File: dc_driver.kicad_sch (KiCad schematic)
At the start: 30 parts, among them J1 Conn_01x02, J10 Conn_01x02, J11 Conn_01x02, J12 Conn_01x02, J13 Conn_01x02, J14 Conn_01x02, J15 Conn_01x02, J2 Conn_01x02, J3 Conn_01x02, J4 Conn_01x02, J5 Conn_01x02, J6 Conn_01x02, J7 Conn_01x02, J8 Conn_01x02, J9 Conn_01x02, U4 MX1508, U5 MX1508, U6 MX1508

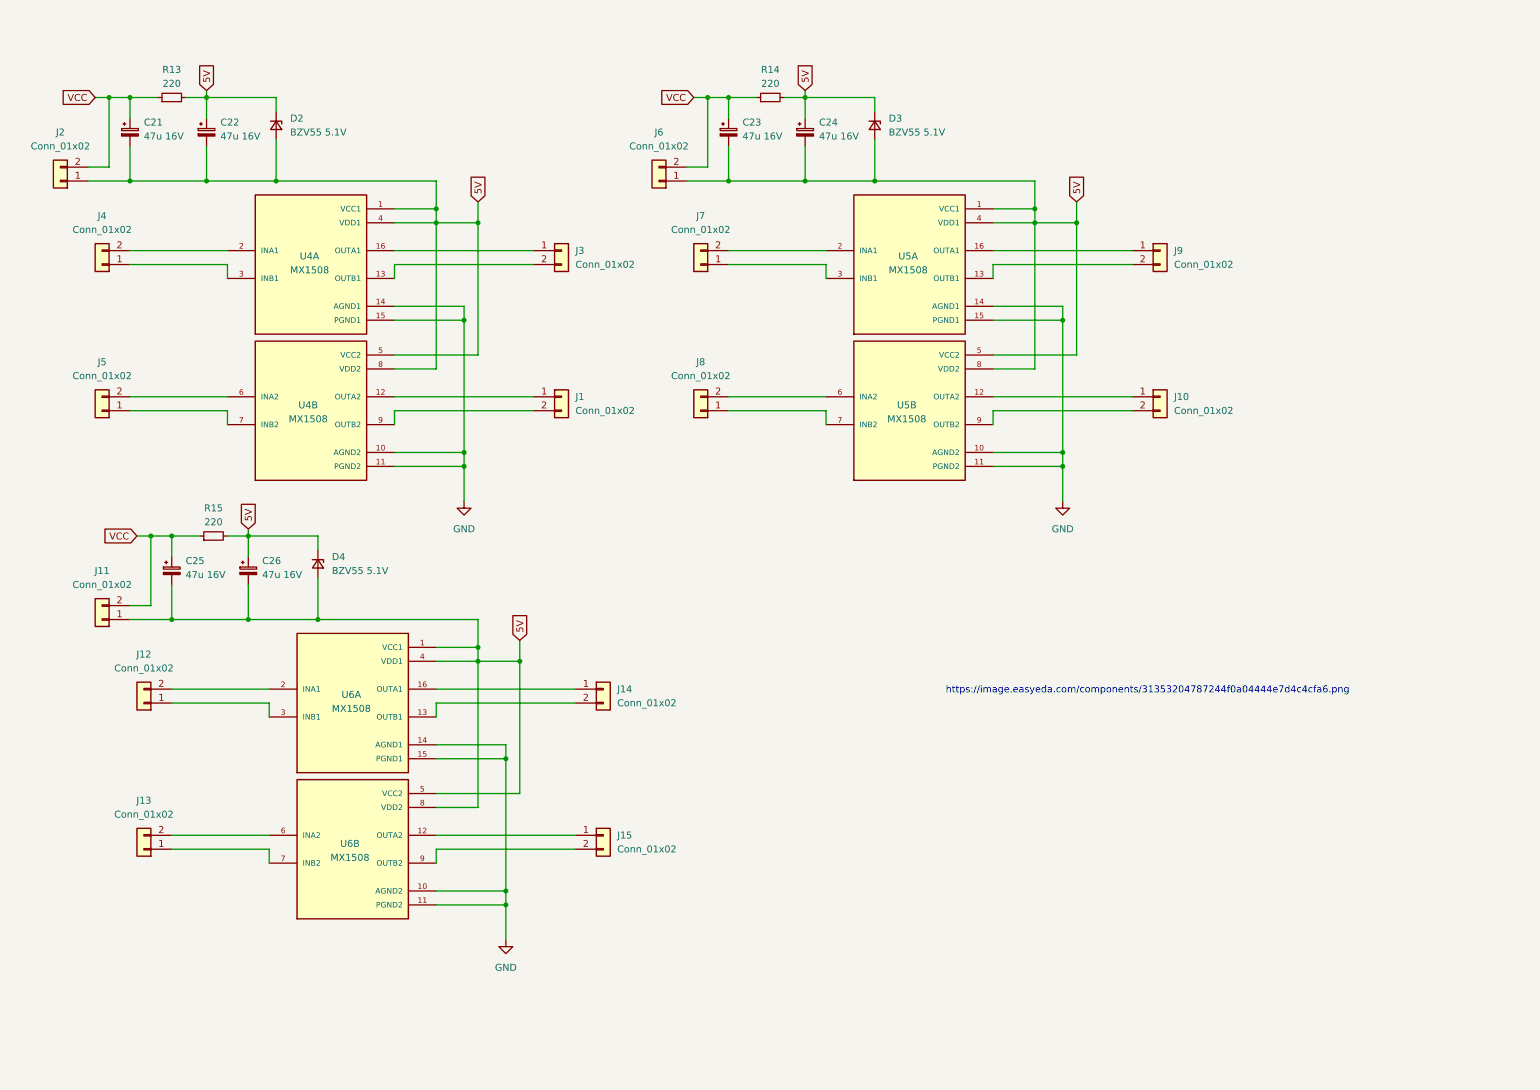
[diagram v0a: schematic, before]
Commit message: stm32 added
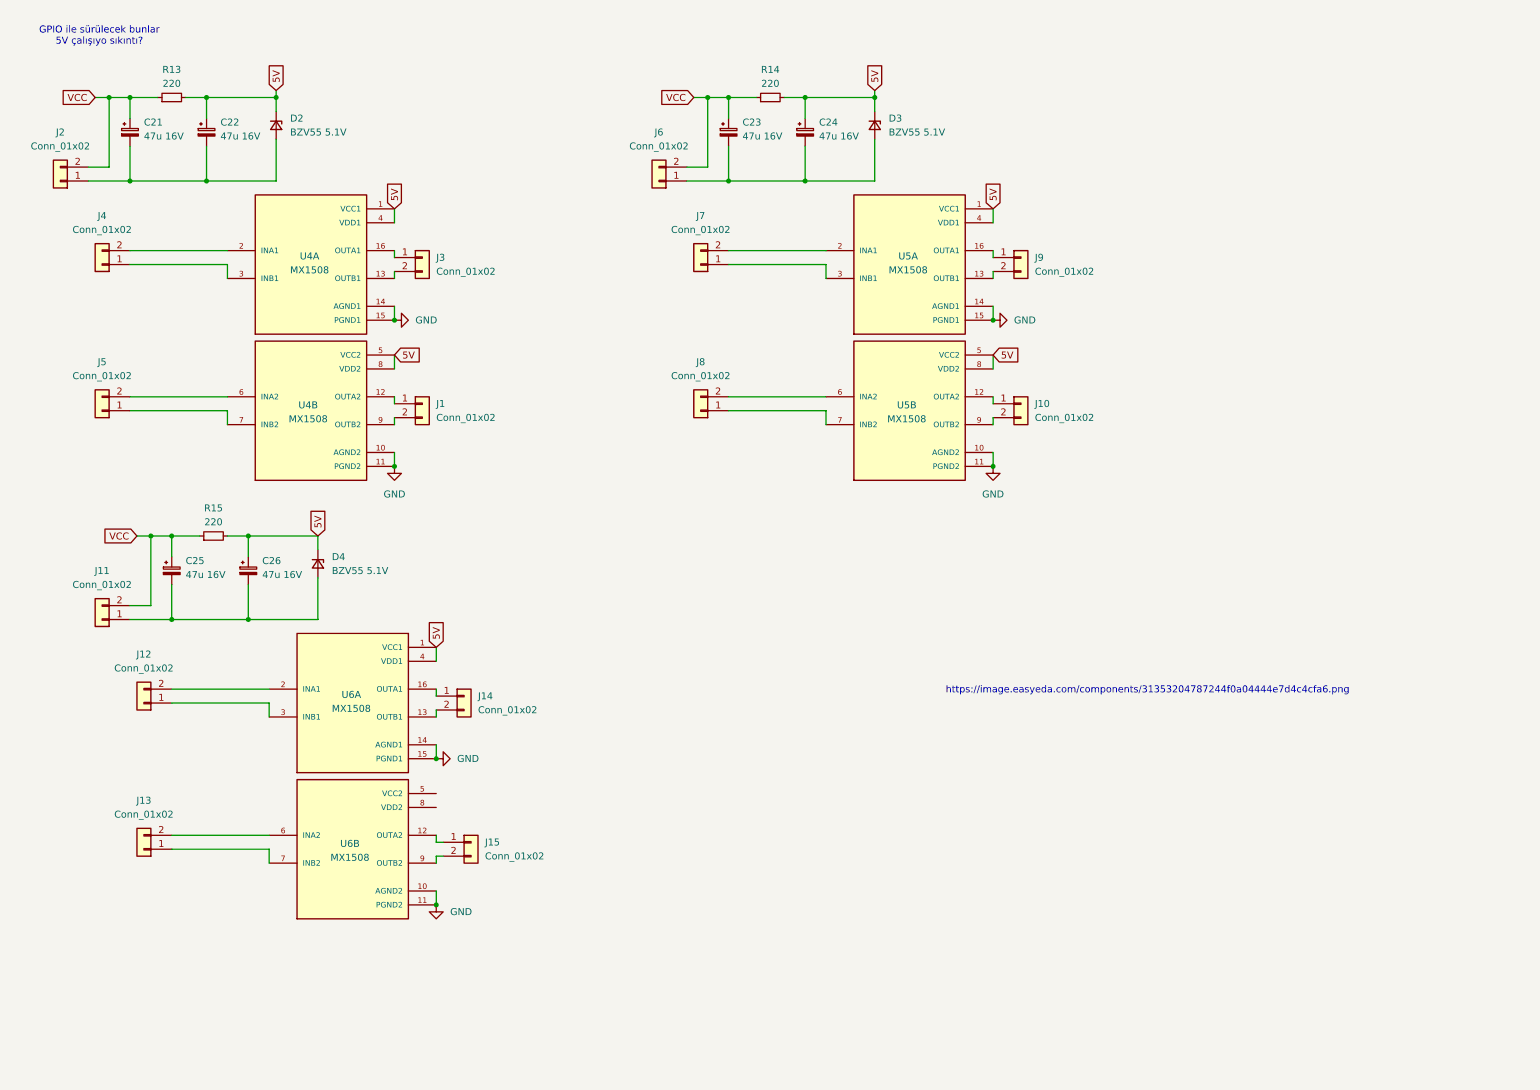
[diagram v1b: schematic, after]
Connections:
- net 5V: no longer C21.2, C22.2, C23.2, C24.2, C25.2, C26.2, D2.2 (A), D3.2 (A), D4.2 (A), J11.1 (Pin_1), J2.1 (Pin_1), J6.1 (Pin_1), U6.5 (VCC2), U6.8 (VDD2)
- new net: C25.2, C26.2, D4.2 (A), J11.1 (Pin_1)
- new net: C23.2, C24.2, D3.2 (A), J6.1 (Pin_1)
- new net: C21.2, C22.2, D2.2 (A), J2.1 (Pin_1)
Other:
- note added: "GPIO ile sürülecek bunlar 5V çalışıyo sıkıntı?"
- moved on the sheet: J1, J10, J14, J15, J3, J9

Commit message: DC motor driver revised
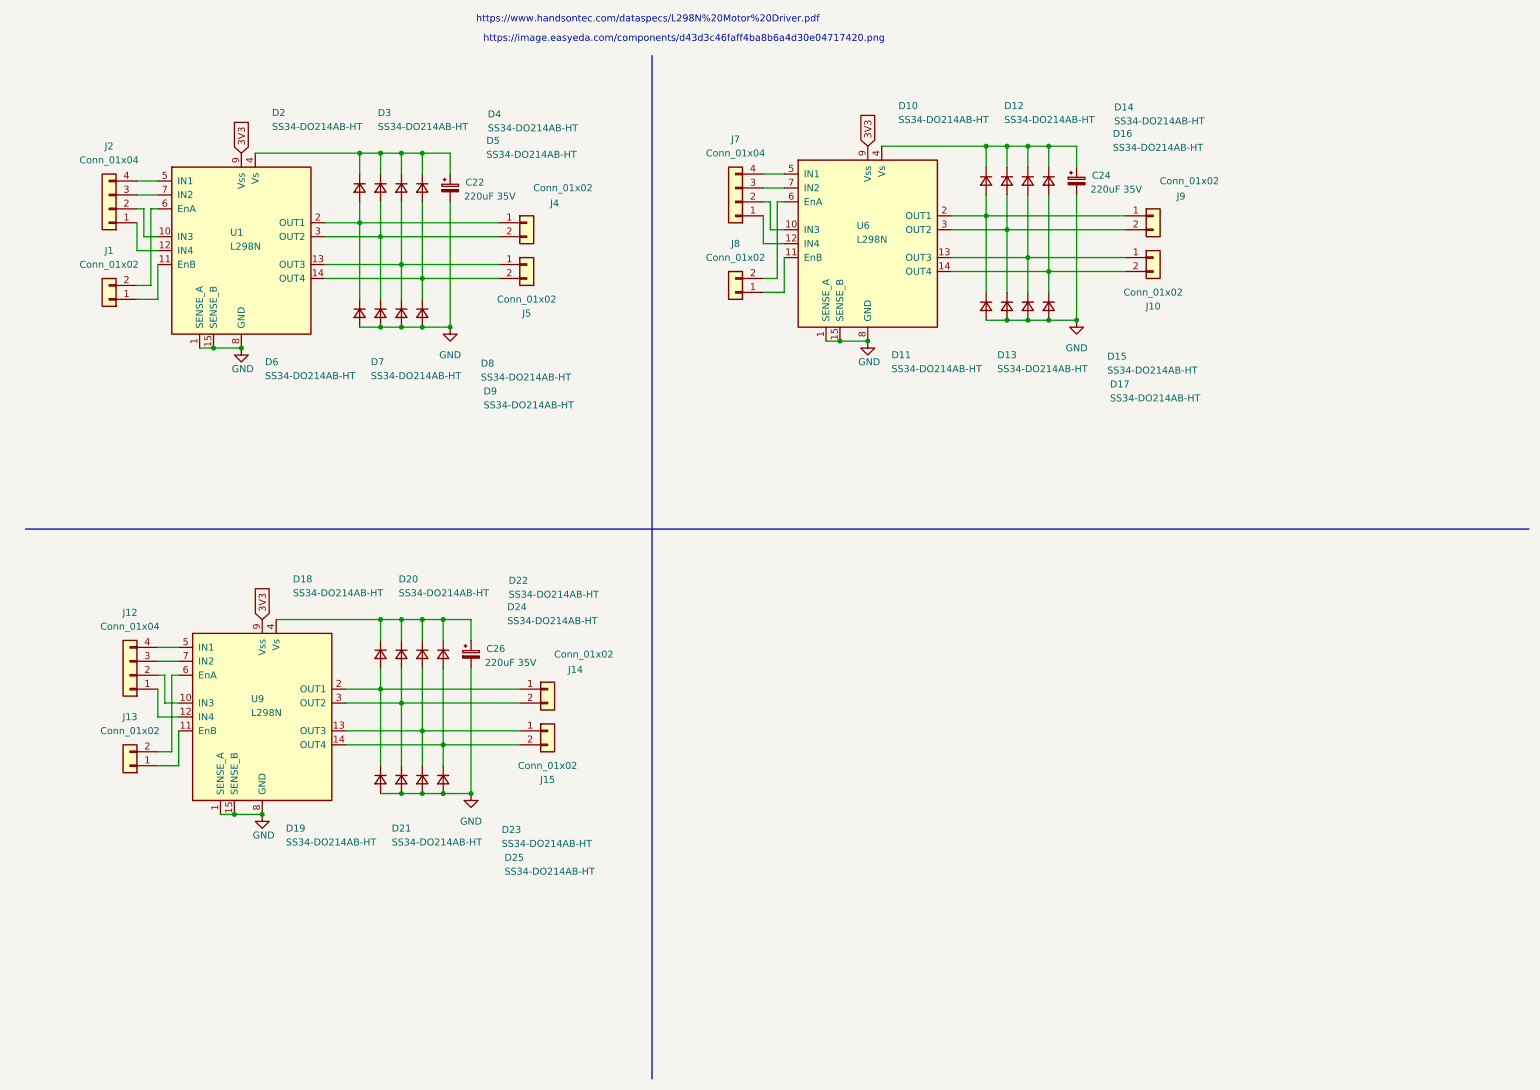
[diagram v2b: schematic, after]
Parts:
- removed C21, C23, C25: 47u 16V, Capacitor_SMD:CP_Elec_5x5.3, symbol Device:C_Polarized_Small
- removed D2, D3, D4: BZV55 5.1V, Diode_SMD:D_SMC, symbol Device:D_Zener_Small
- removed J11, J2, J6: Conn_01x02, symbol Connector_Generic:Conn_01x02
- removed J12, J3, J7: Conn_01x02, Connector_PinHeader_1.00mm:PinHeader_1x02_P1.00mm_Vertical, symbol Connector_Generic:Conn_01x02
- removed R13, R14, R15: 220, Resistor_SMD:R_0805_2012Metric, symbol Device:R_Small
- removed U4, U5, U6: MX1508, MX1508:SOIC127P600X177-16N, symbol MX1508:MX1508
- added D10, D11, D12, D13, D14, D15, D16, D17, D18, D19, D2, D20, D21, D22, D23, D24, D25, D3, D4, D5, D6, D7, D8, D9: SS34-DO214AB-HT, Diode_SMD:D_SMC, symbol Device:D_Small
- added J12, J2, J7: Conn_01x04, symbol Connector_Generic:Conn_01x04
- added U1, U6, U9: L298N, Package_TO_SOT_THT:TO-220-15_P2.54x2.54mm_StaggerOdd_Lead4.58mm_Vertical, symbol Driver_Motor:L298N
- C22, C24: value 47u 16V -> 220uF 35V; footprint Capacitor_SMD:CP_Elec_5x5.3 -> Capacitor_SMD:CP_Elec_8x10.5
- C26: value 47u 16V -> 220uF 35V; footprint Capacitor_SMD:CP_Elec_5x5.3 -> (none)
- J1, J10, J13, J14, J15, J4, J5, J8, J9: footprint Connector_PinHeader_1.00mm:PinHeader_1x02_P1.00mm_Vertical -> (none)
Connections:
- net GND: now also C22.2, C24.2, C26.2, D11.2 (A), D13.2 (A), D15.2 (A), D17.2 (A), D19.2 (A), D21.2 (A), D23.2 (A), D25.2 (A), D6.2 (A), D7.2 (A), D8.2 (A), D9.2 (A), U1.1 (SENSE_A), U1.15 (SENSE_B), U1.8 (GND), U6.1 (SENSE_A), U6.15 (SENSE_B), U6.8 (GND), U9.1 (SENSE_A), U9.15 (SENSE_B), U9.8 (GND)
- net at J15.1 (Pin_1): now also D22.2 (A), D23.1 (K), U9.13 (OUT3)
- net at J15.2 (Pin_2): now also D24.2 (A), D25.1 (K), U9.14 (OUT4)
- net at J10.1 (Pin_1): now also D14.2 (A), D15.1 (K), U6.13 (OUT3)
- net at J10.2 (Pin_2): now also D16.2 (A), D17.1 (K), U6.14 (OUT4)
- net at J4.1 (Pin_1): now also D2.2 (A), D6.1 (K), U1.2 (OUT1)
- net at J4.2 (Pin_2): now also D3.2 (A), D7.1 (K), U1.3 (OUT2)
- net at J5.1 (Pin_1): now also D4.2 (A), D8.1 (K), U1.13 (OUT3)
- net at J5.2 (Pin_2): now also D5.2 (A), D9.1 (K), U1.14 (OUT4)
- net at J13.1 (Pin_1): now also U9.11 (EnB)
- net at J13.2 (Pin_2): now also U9.6 (EnA)
- net at J1.1 (Pin_1): now also U1.11 (EnB)
- net at J1.2 (Pin_2): now also U1.6 (EnA)
- net at J8.2 (Pin_2): now also U6.6 (EnA)
- net at J8.1 (Pin_1): now also U6.11 (EnB)
- net at J14.2 (Pin_2): now also D20.2 (A), D21.1 (K), U9.3 (OUT2)
- net at J14.1 (Pin_1): now also D18.2 (A), D19.1 (K), U9.2 (OUT1)
- net at J9.2 (Pin_2): now also D12.2 (A), D13.1 (K), U6.3 (OUT2)
- net at J9.1 (Pin_1): now also D10.2 (A), D11.1 (K), U6.2 (OUT1)
- removed net 5V: C22.1, C24.1, C26.1
- new net: J2.2 (Pin_2), U1.10 (IN3)
- new net: J2.1 (Pin_1), U1.12 (IN4)
- new net: C22.1, D2.1 (K), D3.1 (K), D4.1 (K), D5.1 (K), U1.4 (Vs)
- new net: J2.4 (Pin_4), U1.5 (IN1)
- new net: J2.3 (Pin_3), U1.7 (IN2)
- new net: C26.1, D18.1 (K), D20.1 (K), D22.1 (K), D24.1 (K), U9.4 (Vs)
- new net: J7.2 (Pin_2), U6.10 (IN3)
- new net: J7.1 (Pin_1), U6.12 (IN4)
- new net: C24.1, D10.1 (K), D12.1 (K), D14.1 (K), D16.1 (K), U6.4 (Vs)
- new net: J7.4 (Pin_4), U6.5 (IN1)
- new net: J7.3 (Pin_3), U6.7 (IN2)
- new net: J12.2 (Pin_2), U9.10 (IN3)
- new net: J12.1 (Pin_1), U9.12 (IN4)
- new net: J12.4 (Pin_4), U9.5 (IN1)
- new net: J12.3 (Pin_3), U9.7 (IN2)
- new net 3V3: U1.9 (Vss), U6.9 (Vss), U9.9 (Vss)
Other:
- note added: "https://image.easyeda.com/components/d43d3c46faff4ba8b6a4d30e04717420.png"
- note added: "https://www.handsontec.com/dataspecs/L298N%20Motor%20Driver.pdf"
- note removed: "GPIO ile sürülecek bunlar 5V çalışıyo sıkıntı?"
- note removed: "https://image.easyeda.com/components/31353204787244f0a04444e7d4c4cfa6.png"
